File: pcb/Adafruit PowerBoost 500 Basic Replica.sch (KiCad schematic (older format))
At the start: 32 parts, among them CN1 USBA, J1 HEADER, J2 PWR OUT, J3 Batería, Q1 MMUN2133LT1G, U1 TPS61090RSAR

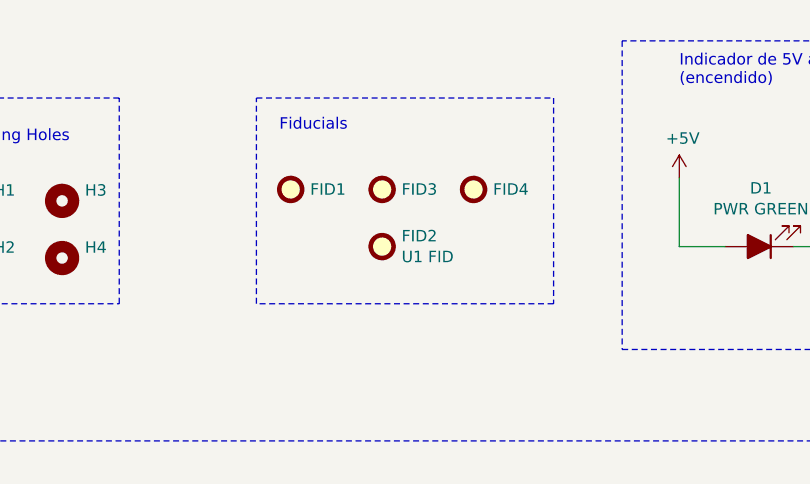
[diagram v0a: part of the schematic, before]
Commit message: Applies Diego Corrections
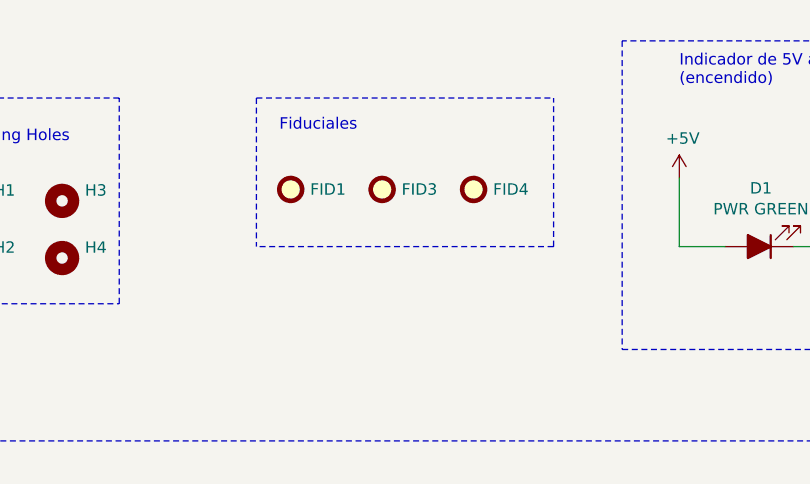
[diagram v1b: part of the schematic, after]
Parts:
- removed FID2: U1 FID, Fiducial:Fiducial_0.5mm_Mask1mm, symbol Mechanical:Fiducial
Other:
- note added: "Fiduciales"
- note removed: "Fiducials"
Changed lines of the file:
@@
 Wire Notes Line
 	4200 1550 3350 1550
-$Comp
-L Mechanical:Fiducial FID2
-U 1 1 616E0E3E
-P 5350 2200
-F 0 "FID2" H 5435 2246 50  0000 L CNN
-F 1 "U1 FID" H 5435 2155 50  0000 L CNN
-F 2 "Fiducial:Fiducial_0.5mm_Mask1mm" H 5350 2200 50  0001 C CNN
-F 3 "~" H 5350 2200 50  0001 C CNN
-	1    5350 2200
-	1    0    0    -1
-$EndComp
-Wire Notes Line
-	4800 2450 4800 1550
 Wire Notes Line
 	4800 1550 6100 1550
 Wire Notes Line
-	6100 1550 6100 2450
-Wire Notes Line
-	6100 2450 4800 2450
+	6100 2200 4800 2200
 Text Notes 4900 1700 0    50   ~ 0
-Fiducials
+Fiduciales
 $Comp
 L Device:Q_PNP_BEC_BRT Q1
@@
 Wire Notes Line
 	8400 4000 11000 4000
+Wire Notes Line
+	6100 2200 6100 1550
+Wire Notes Line
+	4800 1550 4800 2200
 $EndSCHEMATC
